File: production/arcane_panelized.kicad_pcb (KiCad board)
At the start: 2 copper layers, 88.9 x 100.2 mm, 69 parts, among them J1 Conn_01x02, J2 Conn_01x07, SW1 SW_Push, U1 XIAO-nRF52840-SMD

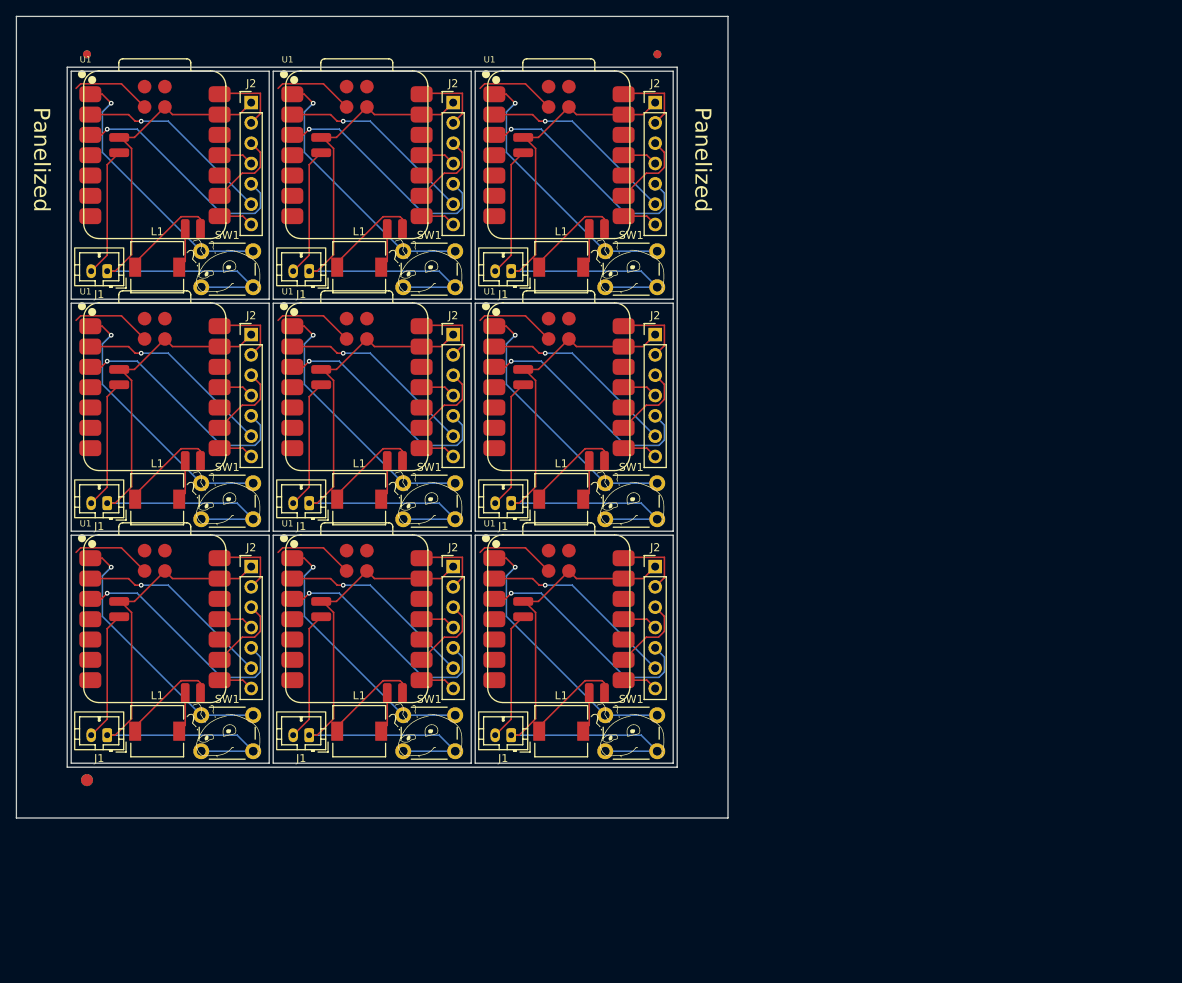
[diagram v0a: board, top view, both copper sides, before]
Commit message: add: gerber files
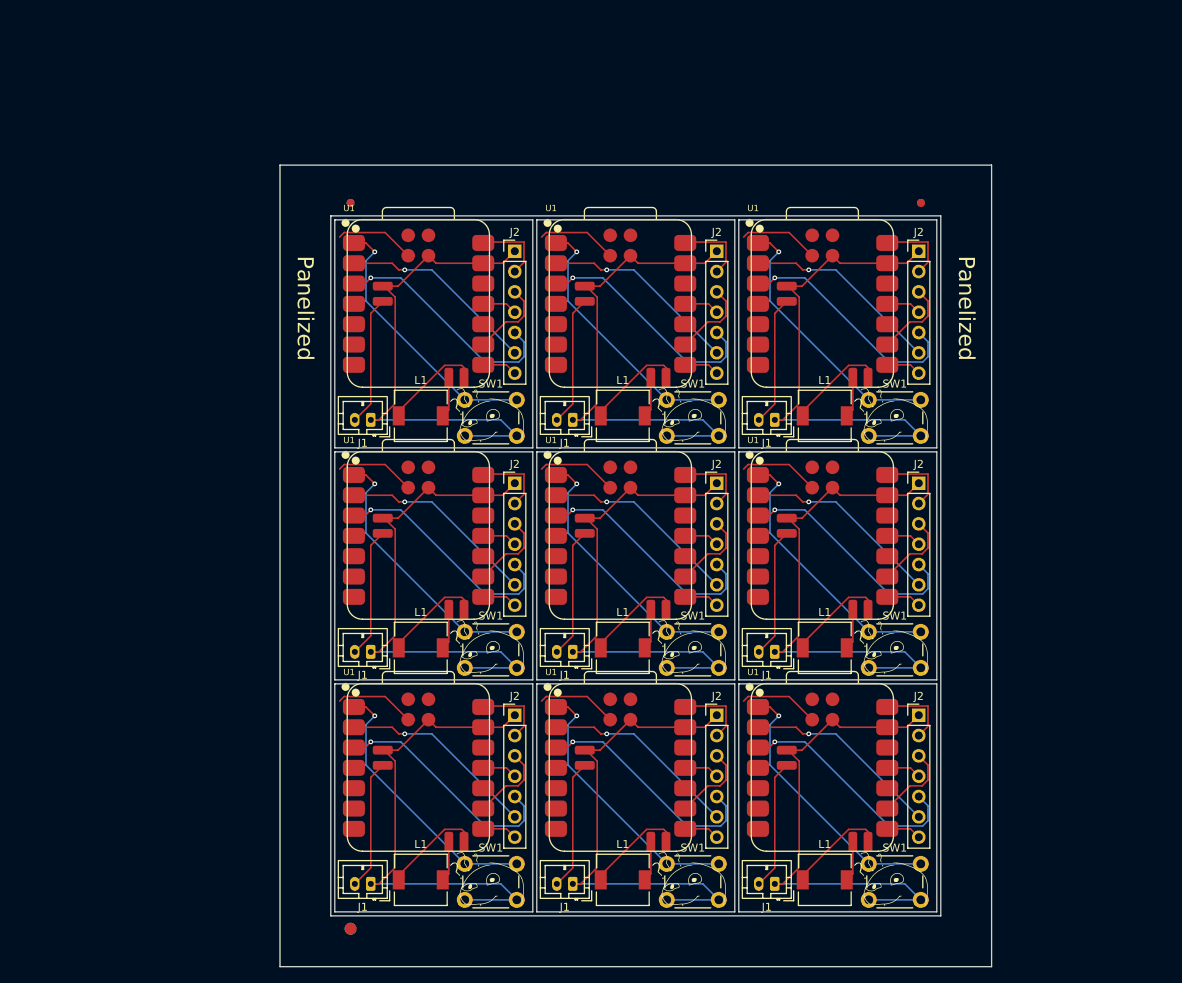
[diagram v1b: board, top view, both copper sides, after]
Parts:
- moved G*** 37.8 mm to (153.4, 136.3)
- moved G*** 37.8 mm to (178.7, 136.3)
- moved G*** 37.8 mm to (128.2, 136.3)
- moved J1 37.8 mm to (138.9, 136.8)
- moved J1 37.8 mm to (164.2, 136.8)
- moved L1 37.8 mm to (145.2, 136.3)
- moved L1 37.8 mm to (170.4, 136.3)
- moved SW1 37.8 mm to (175.9, 134.3)
- moved SW1 37.8 mm to (150.7, 134.3)
- moved ? 37.8 mm to (111.2, 142.4) (x2)
- moved ? 37.8 mm to (111.2, 51.7) (x2)
- moved G*** 37.8 mm to (171.7, 90.6)
- moved G*** 37.8 mm to (146.4, 119.6)
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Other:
- board size 88.9 x 100.2 mm -> 89 x 100.2 mm

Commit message: update: zine, firmware and gerber
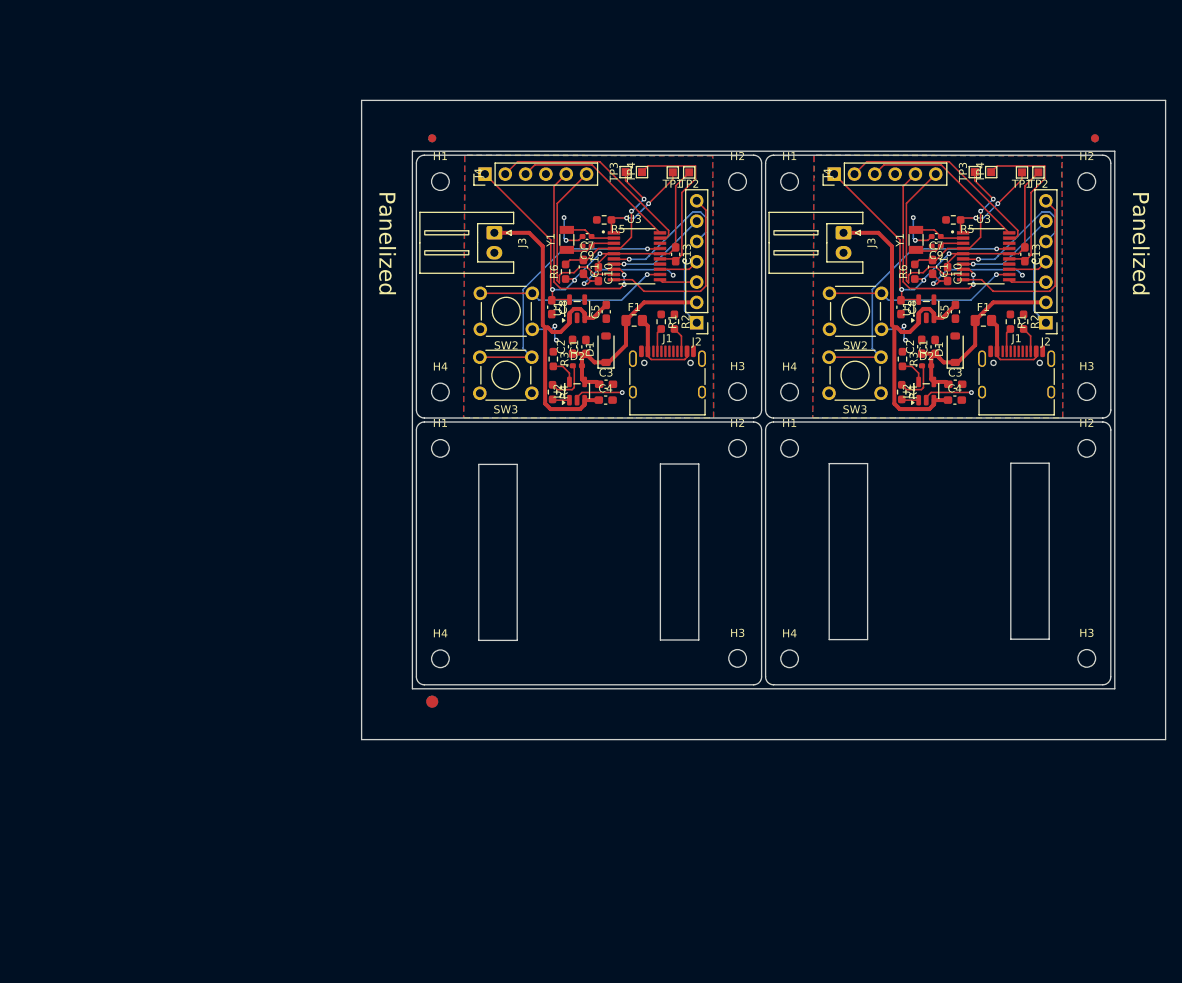
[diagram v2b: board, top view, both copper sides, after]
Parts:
- removed the ? at (111.2, 142.4) (x2)
- removed the ? at (182.5, 51.7) (x2)
- removed the ? at (111.2, 51.7) (x2)
- removed G*** (x18): LOGO, LOGO
- removed the J1 at (138.9, 78.8)
- removed the J1 at (113.7, 136.8)
- removed the J1 at (138.9, 107.8)
- removed the J1 at (113.7, 107.8)
- removed the J1 at (164.2, 78.8)
- removed the J1 at (113.7, 78.8)
- removed the J1 at (164.2, 107.8)
- removed the J1 at (138.9, 136.8)
- removed the J1 at (164.2, 136.8)
- removed the J2 at (182.2, 115.8)
- removed the J2 at (182.2, 57.8)
- removed the J2 at (131.7, 57.8)
- removed the J2 at (156.9, 115.8)
- removed the J2 at (131.7, 86.8)
- removed the J2 at (131.7, 115.8)
- removed the J2 at (156.9, 57.8)
- removed the J2 at (156.9, 86.8)
- removed the J2 at (182.2, 86.8)
- removed L1 (x9): L, Inductor_SMD:L_6.3x6.3_H3
- removed SW1 (x9): SW_Push, Button_Switch_THT:SW_PUSH_6mm
- removed the U1 at (119.7, 122.3)
- removed the U1 at (170.2, 122.3)
- removed the U1 at (144.9, 93.3)
- removed the U1 at (119.7, 64.3)
- removed the U1 at (170.2, 93.3)
- removed the U1 at (119.7, 93.3)
- removed the U1 at (144.9, 64.3)
- removed the U1 at (170.2, 64.3)
- removed the U1 at (144.9, 122.3)
- added ?: , Fiducial_1.5mm_Mask3mm, F.Cu at (121.4, 114.1)
- added ?: , Fiducial_1mm_Mask3mm, F.Cu at (121.4, 43.6)
- added ?: , Fiducial_1mm_Mask3mm, F.Cu at (204.2, 43.6)
- added ?: , Fiducial_1mm_Mask3mm, B.Cu at (121.4, 43.6)
- added ?: , Fiducial_1.5mm_Mask3mm, B.Cu at (121.4, 114.1)
- added ?: , Fiducial_1mm_Mask3mm, B.Cu at (204.2, 43.6)
- added C1: 4.7uf, Capacitor_SMD:C_0603_1608Metric_Pad1.08x0.95mm_HandSolder, F.Cu at (140.6, 69.7)
- added C1: 4.7uf, Capacitor_SMD:C_0603_1608Metric_Pad1.08x0.95mm_HandSolder, F.Cu at (184.2, 69.7)
- added C10: 100uf, Capacitor_SMD:C_0603_1608Metric_Pad1.08x0.95mm_HandSolder, F.Cu at (142.2, 60.6)
- added C10: 100uf, Capacitor_SMD:C_0603_1608Metric_Pad1.08x0.95mm_HandSolder, F.Cu at (185.8, 60.6)
- added C11: 100nf, Capacitor_SMD:C_0603_1608Metric_Pad1.08x0.95mm_HandSolder, F.Cu at (140.3, 59.7)
- added C11: 100nf, Capacitor_SMD:C_0603_1608Metric_Pad1.08x0.95mm_HandSolder, F.Cu at (183.9, 59.7)
- added C13: 100nf, Capacitor_SMD:C_0603_1608Metric_Pad1.08x0.95mm_HandSolder, F.Cu at (151.8, 58.1)
- added C13: 100nf, Capacitor_SMD:C_0603_1608Metric_Pad1.08x0.95mm_HandSolder, F.Cu at (195.5, 58.1)
- added C2: 100nf, Capacitor_SMD:C_0603_1608Metric_Pad1.08x0.95mm_HandSolder, F.Cu at (138.9, 69.7)
- added C2: 100nf, Capacitor_SMD:C_0603_1608Metric_Pad1.08x0.95mm_HandSolder, F.Cu at (182.6, 69.7)
- added C3: 4.7uf, Capacitor_SMD:C_0603_1608Metric_Pad1.08x0.95mm_HandSolder, F.Cu at (143.1, 74.4)
- added C3: 4.7uf, Capacitor_SMD:C_0603_1608Metric_Pad1.08x0.95mm_HandSolder, F.Cu at (186.8, 74.4)
- added C4: 4.7uf, Capacitor_SMD:C_0603_1608Metric_Pad1.08x0.95mm_HandSolder, F.Cu at (143.1, 76.4)
- added C4: 4.7uf, Capacitor_SMD:C_0603_1608Metric_Pad1.08x0.95mm_HandSolder, F.Cu at (186.7, 76.4)
- added C5: 10uf, Capacitor_SMD:C_0603_1608Metric_Pad1.08x0.95mm_HandSolder, F.Cu at (143.1, 65.3)
- added C5: 10uf, Capacitor_SMD:C_0603_1608Metric_Pad1.08x0.95mm_HandSolder, F.Cu at (186.8, 65.3)
- added C7: 22pf, Capacitor_SMD:C_0402_1005Metric_Pad0.74x0.62mm_HandSolder, F.Cu at (140.7, 55.9)
- added C7: 22pf, Capacitor_SMD:C_0402_1005Metric_Pad0.74x0.62mm_HandSolder, F.Cu at (184.4, 55.9)
- added C8: 10uf, Capacitor_SMD:C_0603_1608Metric_Pad1.08x0.95mm_HandSolder, F.Cu at (136.3, 64.8)
- added C8: 10uf, Capacitor_SMD:C_0603_1608Metric_Pad1.08x0.95mm_HandSolder, F.Cu at (180.0, 64.8)
- added C9: 22pf, Capacitor_SMD:C_0402_1005Metric_Pad0.74x0.62mm_HandSolder, F.Cu at (140.7, 57.1)
- added C9: 22pf, Capacitor_SMD:C_0402_1005Metric_Pad0.74x0.62mm_HandSolder, F.Cu at (184.4, 57.1)
- added D1: 5V, Diode_SMD:D_SOD-123, F.Cu at (143.1, 70.0)
- added D1: 5V, Diode_SMD:D_SOD-123, F.Cu at (186.8, 70.0)
- added D2: LED, LED_SMD:LED_0402_1005Metric_Pad0.77x0.64mm_HandSolder, F.Cu at (139.5, 72.1)
- added D2: LED, LED_SMD:LED_0402_1005Metric_Pad0.77x0.64mm_HandSolder, F.Cu at (183.2, 72.1)
- added F1: Polyfuse, Fuse:Fuse_0805_2012Metric_Pad1.15x1.40mm_HandSolder, F.Cu at (146.6, 66.4)
- added F1: Polyfuse, Fuse:Fuse_0805_2012Metric_Pad1.15x1.40mm_HandSolder, F.Cu at (190.3, 66.4)
- added H1: MountingHole, MountingHole:MountingHole_2.2mm_M2, F.Cu at (122.4, 82.4)
- added H1: MountingHole, MountingHole:MountingHole_2.2mm_M2, F.Cu at (122.4, 49.0)
- added H1: MountingHole, MountingHole:MountingHole_2.2mm_M2, F.Cu at (166.1, 82.4)
- added H1: MountingHole, MountingHole:MountingHole_2.2mm_M2, F.Cu at (166.1, 49.0)
- added H2: MountingHole, MountingHole:MountingHole_2.2mm_M2, F.Cu at (159.6, 82.4)
- added H2: MountingHole, MountingHole:MountingHole_2.2mm_M2, F.Cu at (159.6, 49.0)
- added H2: MountingHole, MountingHole:MountingHole_2.2mm_M2, F.Cu at (203.2, 82.4)
- added H2: MountingHole, MountingHole:MountingHole_2.2mm_M2, F.Cu at (203.2, 49.0)
- added H3: MountingHole, MountingHole:MountingHole_2.2mm_M2, F.Cu at (159.6, 108.7)
- added H3: MountingHole, MountingHole:MountingHole_2.2mm_M2, F.Cu at (159.6, 75.3)
- added H3: MountingHole, MountingHole:MountingHole_2.2mm_M2, F.Cu at (203.2, 108.7)
- added H3: MountingHole, MountingHole:MountingHole_2.2mm_M2, F.Cu at (203.2, 75.3)
- added H4: MountingHole, MountingHole:MountingHole_2.2mm_M2, F.Cu at (122.4, 108.7)
- added H4: MountingHole, MountingHole:MountingHole_2.2mm_M2, F.Cu at (122.4, 75.3)
- added H4: MountingHole, MountingHole:MountingHole_2.2mm_M2, F.Cu at (166.1, 108.7)
- added H4: MountingHole, MountingHole:MountingHole_2.2mm_M2, F.Cu at (166.1, 75.3)
- added J1: USB_C_Receptacle_USB2.0_16P, Connector_USB:USB_C_Receptacle_HRO_TYPE-C-31-M-12, F.Cu at (150.8, 74.3)
- added J1: USB_C_Receptacle_USB2.0_16P, Connector_USB:USB_C_Receptacle_HRO_TYPE-C-31-M-12, F.Cu at (194.4, 74.3)
- added J2: Conn_01x07, Connector_PinHeader_2.54mm:PinHeader_1x07_P2.54mm_Vertical, F.Cu at (154.4, 66.7)
- added J2: Conn_01x07, Connector_PinHeader_2.54mm:PinHeader_1x07_P2.54mm_Vertical, F.Cu at (198.1, 66.7)
- added J3: Conn_01x02, Connector_JST:JST_XH_S2B-XH-A_1x02_P2.50mm_Horizontal, F.Cu at (129.1, 55.5)
- added J3: Conn_01x02, Connector_JST:JST_XH_S2B-XH-A_1x02_P2.50mm_Horizontal, F.Cu at (172.8, 55.5)
- added J4: Conn_01x06, Connector_PinHeader_2.54mm:PinHeader_1x06_P2.54mm_Vertical, F.Cu at (128.0, 48.1)
- added J4: Conn_01x06, Connector_PinHeader_2.54mm:PinHeader_1x06_P2.54mm_Vertical, F.Cu at (171.6, 48.1)
- added R1: 5.1K, Resistor_SMD:R_0603_1608Metric_Pad0.98x0.95mm_HandSolder, F.Cu at (150.0, 66.6)
- added R1: 5.1K, Resistor_SMD:R_0603_1608Metric_Pad0.98x0.95mm_HandSolder, F.Cu at (193.7, 66.6)
- added R2: 5.1K, Resistor_SMD:R_0603_1608Metric_Pad0.98x0.95mm_HandSolder, F.Cu at (151.7, 66.6)
- added R2: 5.1K, Resistor_SMD:R_0603_1608Metric_Pad0.98x0.95mm_HandSolder, F.Cu at (195.3, 66.6)
- added R3: 2K, Resistor_SMD:R_0603_1608Metric_Pad0.98x0.95mm_HandSolder, F.Cu at (136.5, 71.2)
- added R3: 2K, Resistor_SMD:R_0603_1608Metric_Pad0.98x0.95mm_HandSolder, F.Cu at (180.2, 71.2)
- added R4: 470E, Resistor_SMD:R_0603_1608Metric_Pad0.98x0.95mm_HandSolder, F.Cu at (136.4, 75.4)
- added R4: 470E, Resistor_SMD:R_0603_1608Metric_Pad0.98x0.95mm_HandSolder, F.Cu at (180.1, 75.4)
- added R5: 10K, Resistor_SMD:R_0603_1608Metric_Pad0.98x0.95mm_HandSolder, F.Cu at (142.9, 53.8)
- added R5: 10K, Resistor_SMD:R_0603_1608Metric_Pad0.98x0.95mm_HandSolder, F.Cu at (186.5, 53.8)
- added R6: 10K, Resistor_SMD:R_0603_1608Metric_Pad0.98x0.95mm_HandSolder, F.Cu at (138.1, 60.3)
- added R6: 10K, Resistor_SMD:R_0603_1608Metric_Pad0.98x0.95mm_HandSolder, F.Cu at (181.7, 60.3)
- added SW2: SW_Push, Button_Switch_THT:SW_TH_Tactile_Omron_B3F-100x, F.Cu at (133.9, 67.5)
- added SW2: SW_Push, Button_Switch_THT:SW_TH_Tactile_Omron_B3F-100x, F.Cu at (177.5, 67.5)
- added SW3: SW_Push, Button_Switch_THT:SW_TH_Tactile_Omron_B3F-100x, F.Cu at (133.8, 75.5)
- added SW3: SW_Push, Button_Switch_THT:SW_TH_Tactile_Omron_B3F-100x, F.Cu at (177.5, 75.5)
- added TP1: TestPoint, TestPoint:TestPoint_Pad_1.0x1.0mm, F.Cu at (151.4, 47.9)
- added TP1: TestPoint, TestPoint:TestPoint_Pad_1.0x1.0mm, F.Cu at (195.1, 47.9)
- added TP2: TestPoint, TestPoint:TestPoint_Pad_1.0x1.0mm, F.Cu at (153.5, 47.9)
- added TP2: TestPoint, TestPoint:TestPoint_Pad_1.0x1.0mm, F.Cu at (197.2, 47.9)
- added TP3: TestPoint, TestPoint:TestPoint_Pad_1.0x1.0mm, F.Cu at (145.6, 47.9)
- added TP3: TestPoint, TestPoint:TestPoint_Pad_1.0x1.0mm, F.Cu at (189.2, 47.9)
- added TP4: TestPoint, TestPoint:TestPoint_Pad_1.0x1.0mm, F.Cu at (147.6, 47.9)
- added TP4: TestPoint, TestPoint:TestPoint_Pad_1.0x1.0mm, F.Cu at (191.2, 47.9)
- added U1: XC6220B331MR, Package_TO_SOT_SMD:SOT-23-5, F.Cu at (139.5, 64.9)
- added U1: XC6220B331MR, Package_TO_SOT_SMD:SOT-23-5, F.Cu at (183.1, 64.9)
- added U2: MCP73831-2-OT, Package_TO_SOT_SMD:SOT-23-5, F.Cu at (183.1, 75.2)
- added U2: MCP73831-2-OT, Package_TO_SOT_SMD:SOT-23-5, F.Cu at (139.5, 75.2)
- added U3: STM32L031F6P6, STM32:SOP65P640X120-20N, F.Cu at (147.0, 58.4)
- added U3: STM32L031F6P6, STM32:SOP65P640X120-20N, F.Cu at (190.6, 58.4)
- added Y1: Crystal, Crystal:Crystal_SMD_3215-2Pin_3.2x1.5mm, F.Cu at (138.2, 56.3)
- added Y1: Crystal, Crystal:Crystal_SMD_3215-2Pin_3.2x1.5mm, F.Cu at (181.9, 56.3)
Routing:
- net GND: track 575.8 -> 122.6 mm, vias 0 -> 16
- net Net-(U1-P0.02_A0_D0): track 302.8 -> 0.00 mm, vias 9 -> 0
- net RST: track 267.2 -> 0.00 mm, vias 9 -> 0
- net DC: track 222.7 -> 0.00 mm, vias 9 -> 0
- net Net-(J1-Pin_2): track 146.4 -> 0.00 mm
- net Net-(U1-NFC2): track 112.4 -> 0.00 mm
- net +3.3V: track 0.00 -> 106.4 mm, vias 0 -> 6
- net /V_{BAT}: track 0.00 -> 94.8 mm
- net CLK: track 90.6 -> 0.00 mm
- net unconnected-(U1-RESET-Pad21): track 90.1 -> 0.00 mm
- net Net-(U3-PA9): track 0.00 -> 69.2 mm, vias 0 -> 2
- net /SWDIO: track 0.00 -> 52.9 mm
- net /UART TX: track 0.00 -> 52.6 mm, vias 0 -> 4
- net Net-(U3-PA6): track 0.00 -> 48.2 mm, vias 0 -> 2
- net /UART RX: track 0.00 -> 47.5 mm
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- added copper zone on B.Cu, net GND
- added copper zone on F.Cu, net GND
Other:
- board size 89 x 100.2 mm -> 100.5 x 79.9 mm
- board text removed: "ARCANE"
